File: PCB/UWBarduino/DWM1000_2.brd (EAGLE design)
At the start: 33.1 x 76.3 mm, 11 parts, among them IC1 DWM1000

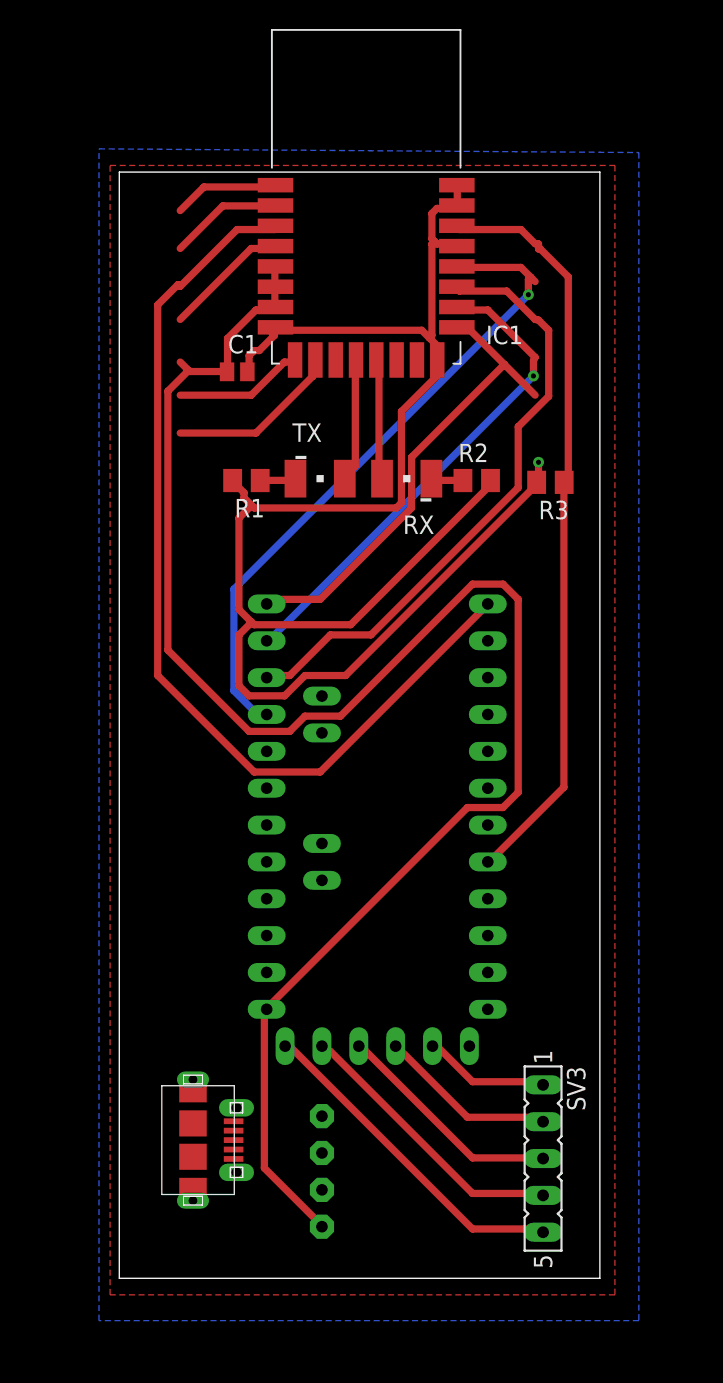
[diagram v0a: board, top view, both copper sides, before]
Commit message: knas
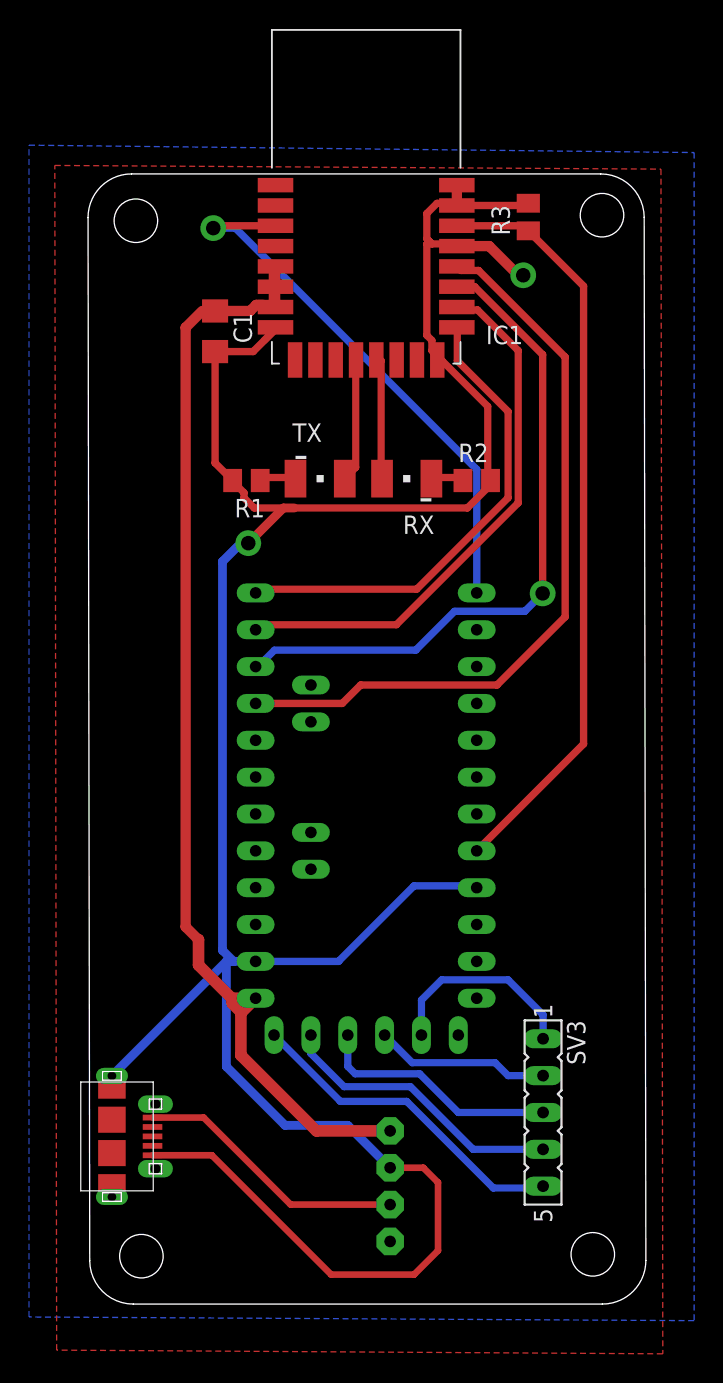
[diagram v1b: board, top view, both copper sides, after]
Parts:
- C1: device eagle-ltspice:C0504 -> eagle-ltspice:C1206
- moved R3 18.4 mm to (31.5, 25.7), turned to 90 degrees
- moved U$1 5.59 mm to (2.79, -37.7)
- moved C1 3.18 mm to (9.91, 17.8), turned to 270 degrees
- moved SV3 3.18 mm to (32.5, -36.1)
- moved U$3 3.09 mm to (18.2, -41.1), turned to 90 degrees
- moved U$2 1.08 mm to (19.1, -15.5)
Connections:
- net GND: now also U$1.CASING1
- net N$3: now also U$1.CASING2; no longer U$1.CASING1
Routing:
- net GND: track 117.6 -> 190.6 mm, vias 1 -> 2
- net 3.3: track 117.5 -> 80.8 mm
- net RST: track 66.5 -> 38.0 mm, vias 0 -> 1
- net 5V: track 0.00 -> 18.9 mm
- net SPIPOL: track 12.0 -> 0.00 mm
- net SPIPHA: track 8.94 -> 0.00 mm
- net SYNC: track 8.72 -> 0.00 mm
- net WAKE: track 7.79 -> 0.00 mm
- net EXT: track 7.33 -> 0.00 mm
- net CLK: track 45.8 -> 51.8 mm, vias 1 -> 0
- net PGND: track 8.70 -> 14.0 mm
- net MISO: track 42.1 -> 46.6 mm, vias 0 -> 1
- net MOSI: track 34.1 -> 37.8 mm, vias 1 -> 0
- net PRX: track 15.9 -> 17.1 mm
- net CS: track 32.6 -> 33.3 mm
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- added copper zone on layer 1, net GND
- removed copper zone on layer 1, net N$4
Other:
- board size 33.1 x 76.3 mm -> 38.5 x 77.9 mm
- board text added: "GND"
- board text added: "Mikael & Filip"
- board text added: "Power in"
- board text added: "Prog in"
- board text added: "RST"
- board text added: "RX"
- board text added: "TX"
- board text added: "VCC"
